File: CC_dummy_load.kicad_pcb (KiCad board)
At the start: 2 copper layers, 120 x 79.8 mm, 58 parts, among them P1 CONN_01X02, P2 12vFAN, P3 CONN_01X09, P4 LOAD, Q1 Darl_NPN, Q2 IRF540N, U1 LM324N, U2 MCP4921-E/P, U3 LM35

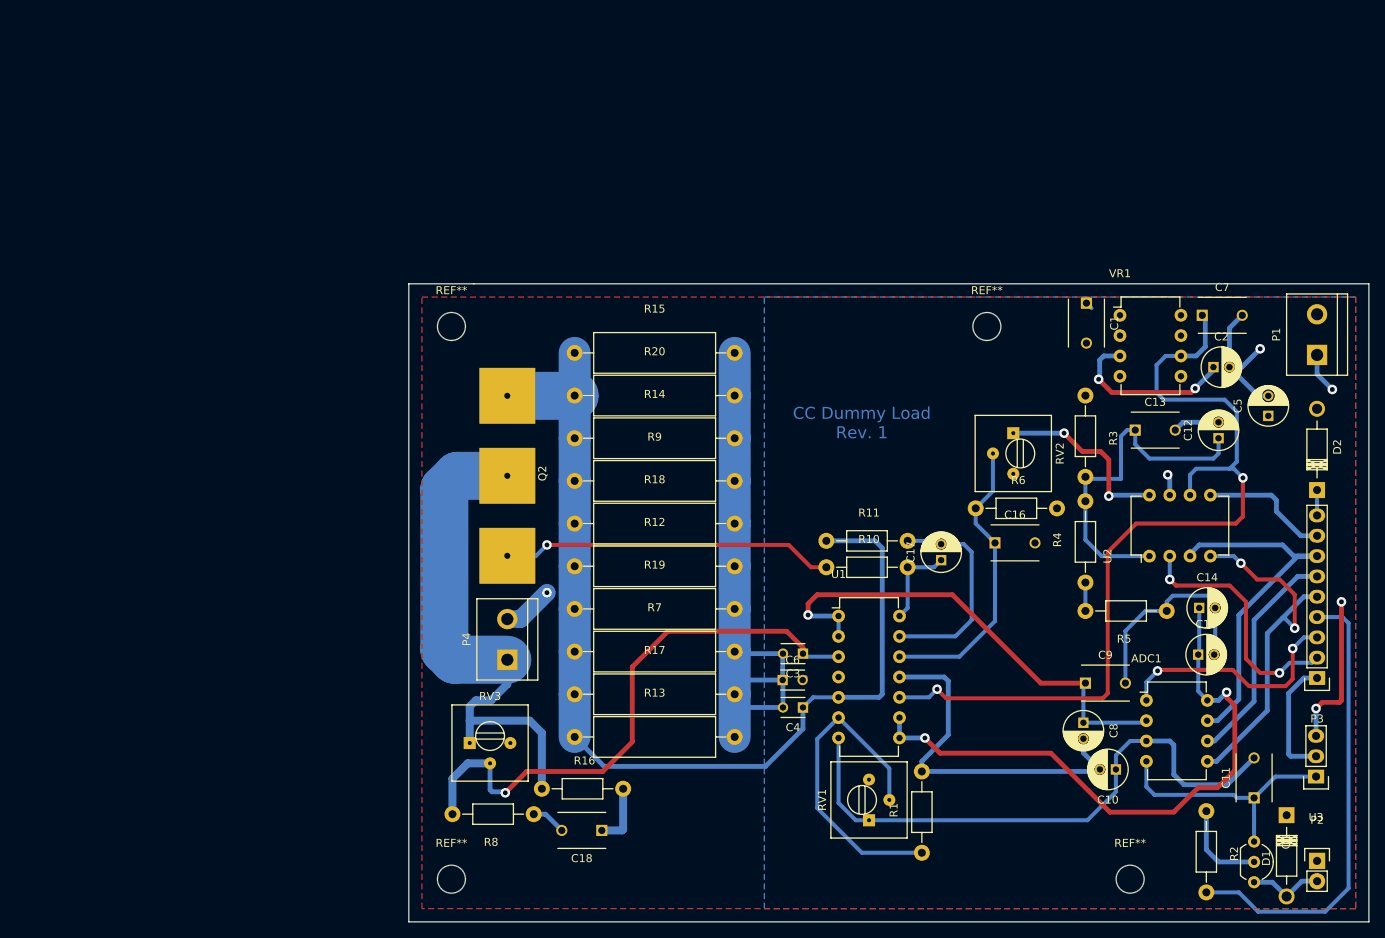
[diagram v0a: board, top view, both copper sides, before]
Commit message: rev 2
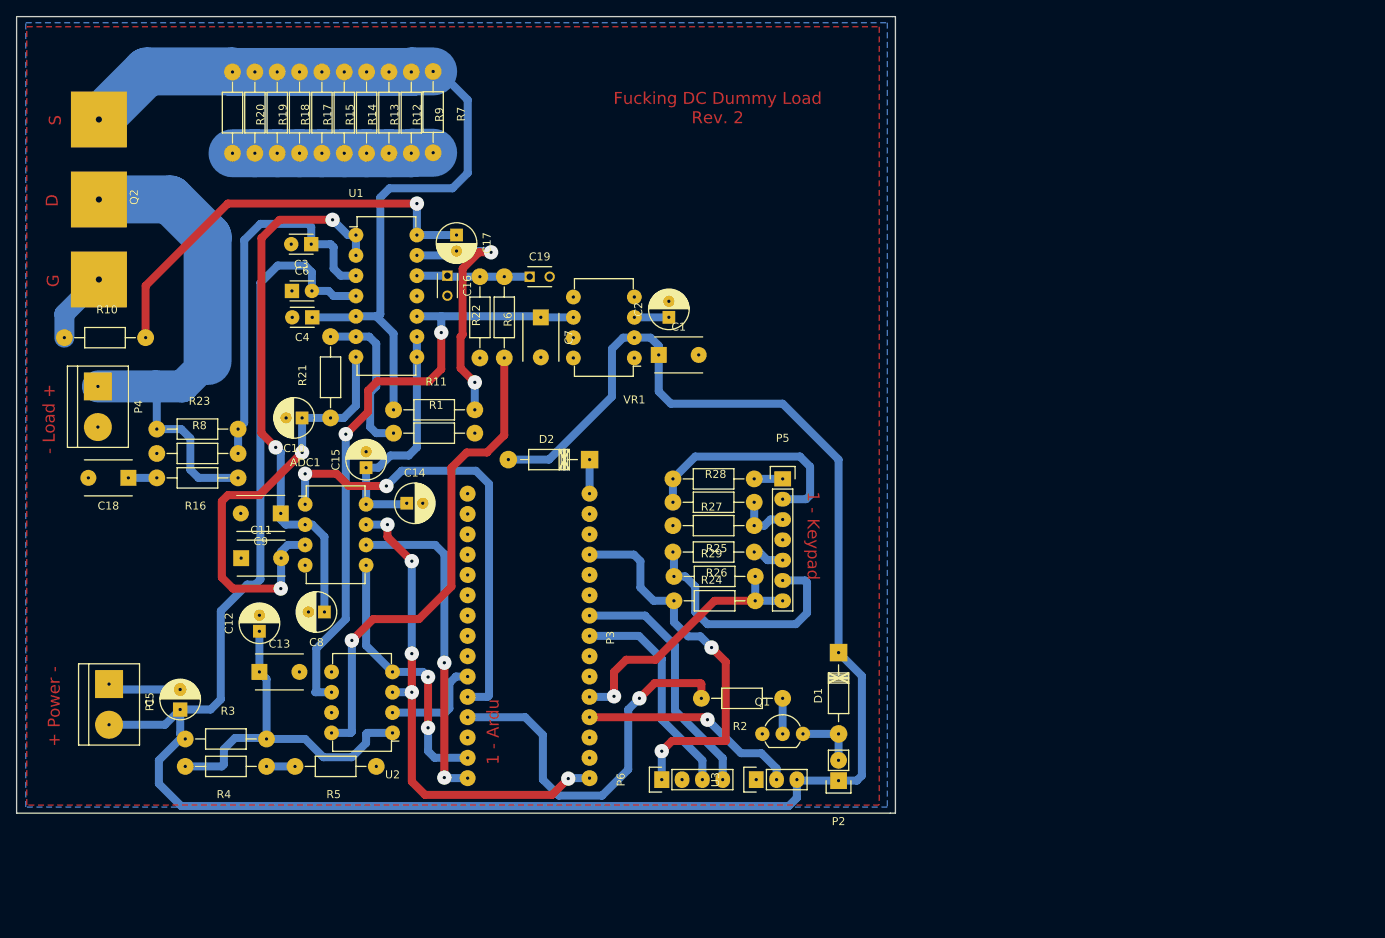
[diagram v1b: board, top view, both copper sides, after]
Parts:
- removed REF** (x4): MountingHole_3-5mm, Mounting_Holes:MountingHole_3-5mm
- removed RV1, RV3: POT, Potentiometers:Potentiometer_Trimmer-Suntan-TSR-3386P
- removed RV2: 10k, Potentiometers:Potentiometer_Trimmer-Suntan-TSR-3386P
- added C19: 150pF, Capacitors_ThroughHole:C_Disc_D3_P2.5, F.Cu at (102.2, 64.1)
- added P5: KeyPad, Pin_Headers:Pin_Header_Straight_1x07, F.Cu at (133.9, 89.4)
- added P6: LCD_I2C, Pin_Headers:Pin_Header_Straight_1x04, F.Cu at (118.7, 127.0)
- added R21: 9.09k, Resistors_ThroughHole:Resistor_Horizontal_RM10mm, F.Cu at (77.3, 76.7)
- added R22: 9.09k, Resistors_ThroughHole:Resistor_Horizontal_RM10mm, F.Cu at (99.1, 69.2)
- added R23: 10k, Resistors_ThroughHole:Resistor_Horizontal_RM10mm, F.Cu at (60.7, 83.2)
- added R24: 22k, Resistors_ThroughHole:Resistor_Horizontal_RM10mm, F.Cu at (125.2, 98.6)
- added R25: 3.3k, Resistors_ThroughHole:Resistor_Horizontal_RM10mm, F.Cu at (125.3, 101.6)
- added R26: 22k, Resistors_ThroughHole:Resistor_Horizontal_RM10mm, F.Cu at (125.3, 104.6)
- added R27: 6.8k, Resistors_ThroughHole:Resistor_Horizontal_RM10mm, F.Cu at (125.2, 89.4)
- added R28: 6.8k, Resistors_ThroughHole:Resistor_Horizontal_RM10mm, F.Cu at (125.2, 92.3)
- added R29: 4.7k, Resistors_ThroughHole:Resistor_Horizontal_RM10mm, F.Cu at (125.2, 95.2)
- C16: value 100n -> 150pF; footprint Capacitors_ThroughHole:C_Disc_D6_P5 -> Capacitors_ThroughHole:C_Disc_D3_P2.5
- C17: value 22n -> 8.2nF
- C3, C4: value C -> 100n
- P3: value CONN_01X09 -> Arduino_Nano; footprint Pin_Headers:Pin_Header_Straight_1x09 -> arduino:Nano
- R12, R13, R14, R15, R17, R18, R19, R20, R7, R9: footprint Resistors_ThroughHole:Resistor_Horizontal_RM20mm -> Resistors_ThroughHole:Resistor_Horizontal_RM10mm
- R8: value 1k -> 2k
- moved P1 157.9 mm to (49.7, 117.6), turned to 270 degrees
- moved C5 140.9 mm to (58.5, 118.2)
- moved C11 130.1 mm to (66.2, 99.3), turned to 0 degrees
- moved C12 122.3 mm to (68.5, 108.5)
- moved R3 113.9 mm to (64.3, 121.9), turned to 0 degrees
- moved C13 113.6 mm to (68.5, 113.5)
- moved R4 111.0 mm to (64.3, 125.3), turned to 180 degrees
- moved C10 110.8 mm to (73.8, 81.8)
- moved ADC1 108.0 mm to (74.2, 92.6)
- moved C15 106.6 mm to (81.8, 88.0), turned to 90 degrees
- moved C9 102.8 mm to (71.1, 93.7), turned to 180 degrees
- moved R5 100.7 mm to (78.0, 125.3)
- moved C14 99.9 mm to (86.9, 92.5)
- moved R10 99.5 mm to (49.1, 71.8)
- moved P3 99.1 mm to (101.7, 109.0), turned to 90 degrees
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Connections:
- P3 pad 1: ARDU-A0 -> ARDU-P12
- P3 pad 2: ARDU-P07 -> ARDU-P11
- P3 pad 3: ARDU-P08 -> Net-(P3-Pad3)
- P3 pad 5: ARDU-P11 -> ARDU-P08
- P3 pad 6: ARDU-P12 -> ARDU-P07
- P3 pad 7: ARDU-P13 -> Net-(P3-Pad7)
- P3 pad 8: GND -> Net-(P3-Pad8)
- P3 pad 9: Net-(D2-Pad1) -> Net-(P3-Pad9)
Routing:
- net VCC: track 20.8 -> 290.6 mm, vias 2 -> 0
- net GND: track 239.2 -> 34.3 mm, vias 4 -> 0
- net ARDU-5v: track 0.00 -> 48.1 mm, vias 0 -> 2
- net Net-(ADC1-Pad8): track 75.6 -> 30.9 mm, vias 2 -> 0
- net Net-(C17-Pad1): track 11.1 -> 53.5 mm, vias 0 -> 1
- net Net-(R22-Pad1): track 23.0 -> 62.1 mm, vias 2 -> 1
- net ARDU-A1: track 0.00 -> 33.9 mm, vias 0 -> 1
- net Net-(Q2-Pad1): track 43.0 -> 9.06 mm, vias 1 -> 0
- net VREF: track 111.4 -> 79.2 mm
- net Net-(P5-Pad6): track 0.00 -> 31.8 mm
- net Net-(P3-Pad24): track 0.00 -> 31.5 mm
- net Net-(P5-Pad2): track 0.00 -> 28.9 mm
- net ARDU-P08: track 29.9 -> 58.1 mm
- net Net-(P3-Pad23): track 0.00 -> 27.4 mm
- net ADC-VIN: track 72.6 -> 47.3 mm, vias 1 -> 0
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- added copper zone on B.Cu, net GND
- removed copper zone on B.Cu, net VCC
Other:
- board size 120 x 79.8 mm -> 109.9 x 99.6 mm
- net class Default: clearance 0.2 -> 0.3; trace_width 0.25 -> 0.6
- rule trace_clearance: 0.2 -> 0.3
- rule trace_min: 0.2 -> 0.6
- rule via_min_size: 0.4 -> 1
- board text added: "+ Power -"
- board text added: "- Load +"
- board text added: "1 - Ardu"
- board text added: "1 - Keypad"
- board text added: "D"
- board text added: "Fucking DC Dummy Load Rev. 2"
- board text added: "G"
- board text added: "S"
- board text removed: "CC Dummy Load Rev. 1"
